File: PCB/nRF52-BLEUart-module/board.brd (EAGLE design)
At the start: 40 x 16 mm, 2 parts, among them J1 USB-A_PTH_MALE, U1 NRF52832

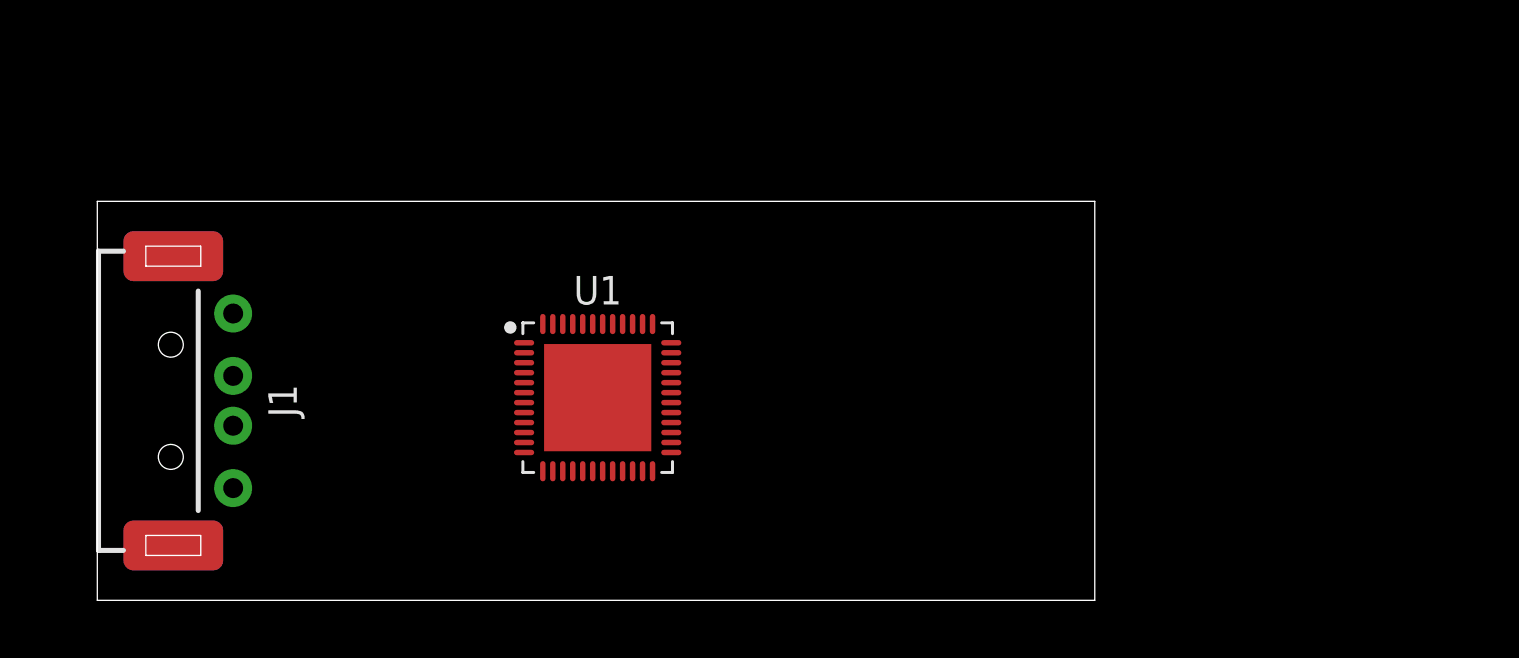
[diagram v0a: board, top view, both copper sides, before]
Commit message: PCB update
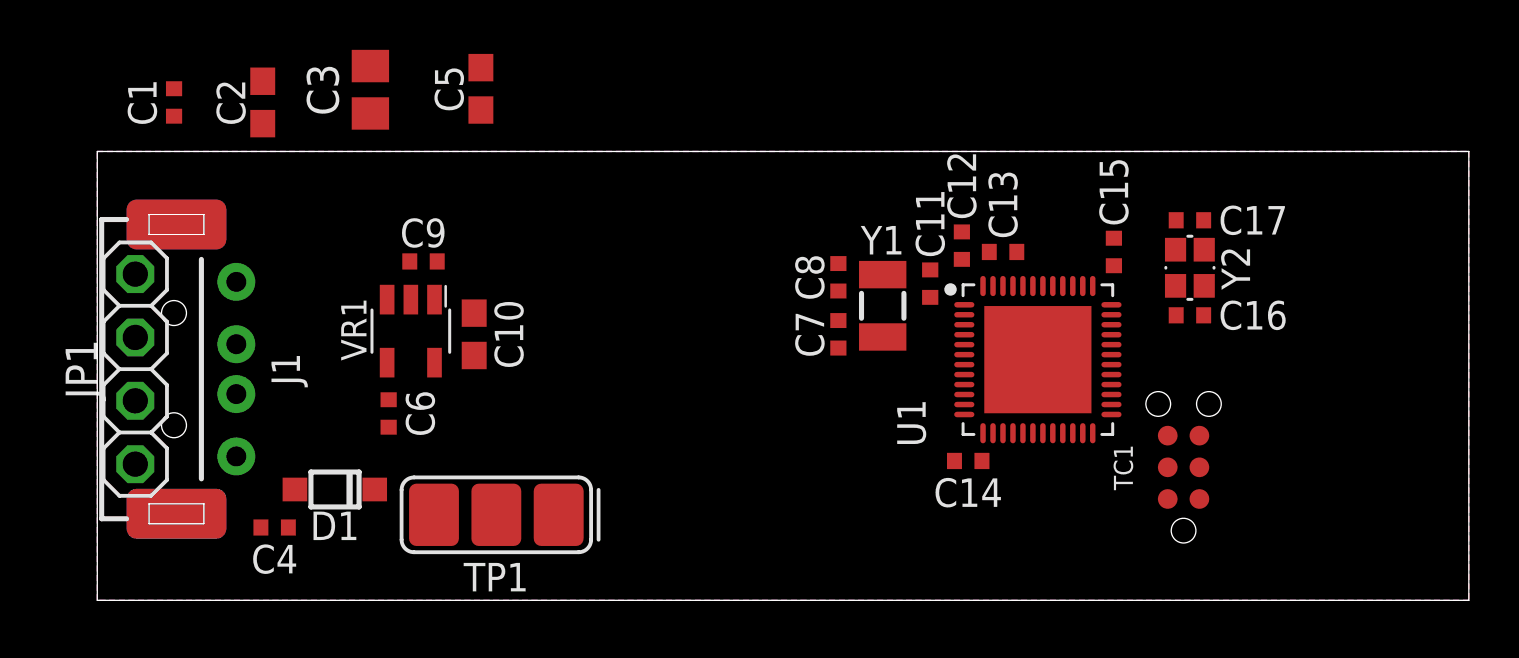
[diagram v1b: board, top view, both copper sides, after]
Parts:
- added C1: 0402, angrypig7-RCL:C0402
- added C10: 2.2uF, angrypig7-RCL:C0603
- added C11, C13, C14, C15, C4, C6: 100nF, angrypig7-RCL:C0402
- added C12: 4.7uF, angrypig7-RCL:C0402
- added C16, C17, C7, C8: 12pF, angrypig7-RCL:C0402
- added C2: 0603, angrypig7-RCL:C0603
- added C3: 0805, angrypig7-RCL:C0805
- added C5: 10uF, angrypig7-RCL:C0603
- added C9: 1uF, angrypig7-RCL:C0402
- added D1: B5819W, angrypig7-Diodes:SOD-123
- added JP1: (no value), angrypig7-Connectors-PinHeads:1X04
- added TC1: TC2030-IDC-NL, angrypig7-Connectors-Programming:TC2030-IDC-NL
- added TP1: TEST-POINT-3, angrypig7-Tests:PAD-3X-RECT-SILK
- added VR1: AP2210K-3.3TRG, angrypig7-IC-Power:SOT-23-5
- added Y1: 32.768kHz, angrypig7-Clocks:CRYSTAL-SMD-3.2X1.5MM
- added Y2: 32MHz_2016, angrypig7-Clocks:CRYSTAL-SMD-2.0X1.6MM
- moved U1 17.7 mm to (37.7, 9.65)
- moved J1 1.28 mm to (3.17, 9.27)
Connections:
- removed net VBUS: J1.VBUS
- new net 3V3: C10.1, C12.1, C14.1, C15.1, TC1.1, TP1.P$2, U1.13, U1.36, U1.48, VR1.5
- new net 5V: C9.1, D1.C, TP1.P$3, VR1.1, VR1.3
- new net N$1: C8.2, U1.2, Y1.P$2
- new net N$2: C4.1, D1.A, J1.VBUS
- new net N$3: C6.1, VR1.4
- new net N$4: C7.2, U1.3, Y1.P$1
- new net N$5: C11.1, U1.1
- new net N$6: U1.30
- new net N$7: C13.1, U1.46
- new net N$8: C17.1, U1.35, Y2.3
- new net N$9: C16.1, U1.34, Y2.1
- new net NRST: TC1.3, U1.24
- new net SWDCLK: TC1.4, U1.25
- new net SWDIO: TC1.2, U1.26
- new net SWO: TC1.6, U1.21
- new net USB_D_N: J1.D-
- new net USB_D_P: J1.D+
- net GND: now also C10.2, C11.2, C12.2, C13.2, C14.2, C15.2, C16.2, C17.2, C4.2, C6.2, C7.1, C8.1, C9.2, J1.SHIELD@0, J1.SHIELD@1, J1.SHIELD@2, J1.SHIELD@3, TC1.5, TP1.P$1, U1.45, VR1.2, Y2.2, Y2.4
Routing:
- added copper zone on layer 1, net GND
- added copper zone on layer 16, net GND
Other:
- board size 40 x 16 mm -> 55 x 18 mm
